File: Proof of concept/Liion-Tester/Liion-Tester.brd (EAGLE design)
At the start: 100 x 80 mm, 24 parts, among them Q2 SI4403DDY-T1-GE3, U1 1042, U2 NCP1854FCCT1G, U3 BQ27427YZFR

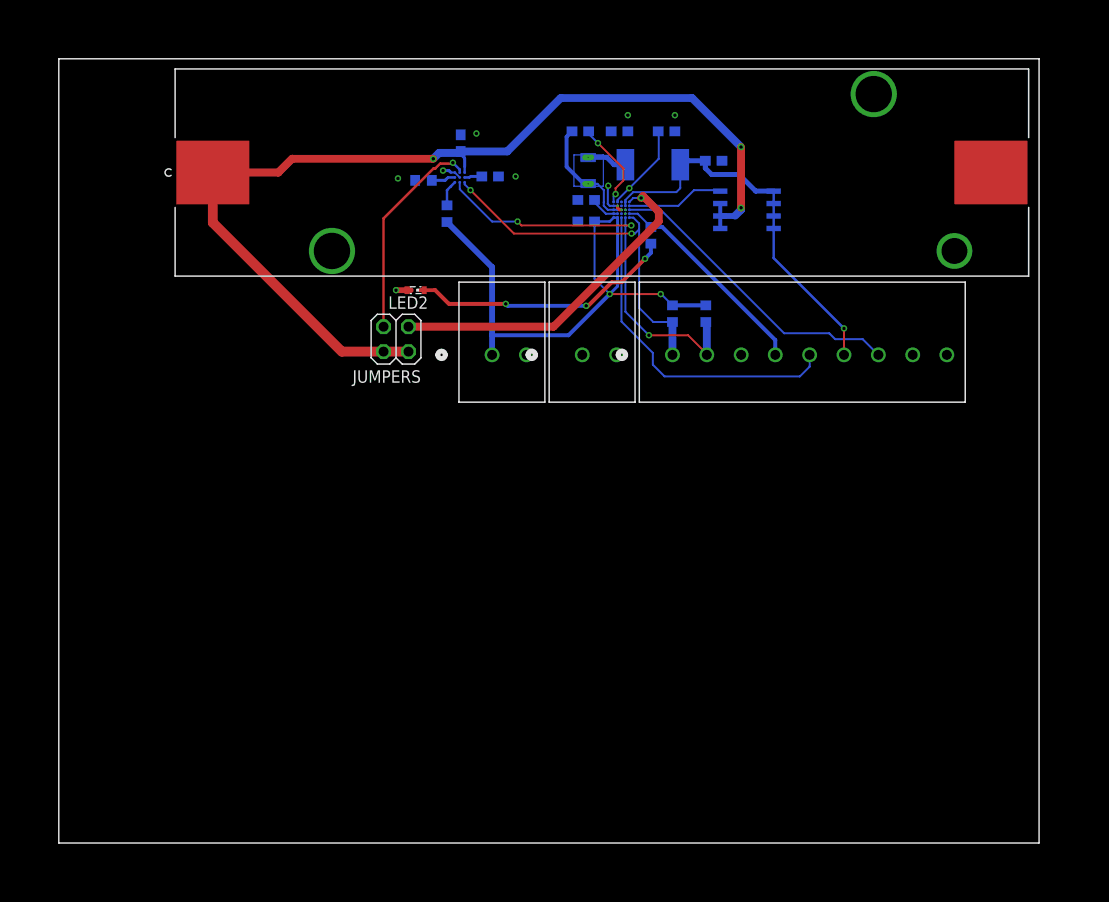
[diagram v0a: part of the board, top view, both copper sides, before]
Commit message: Finished .brd with changes in schematic
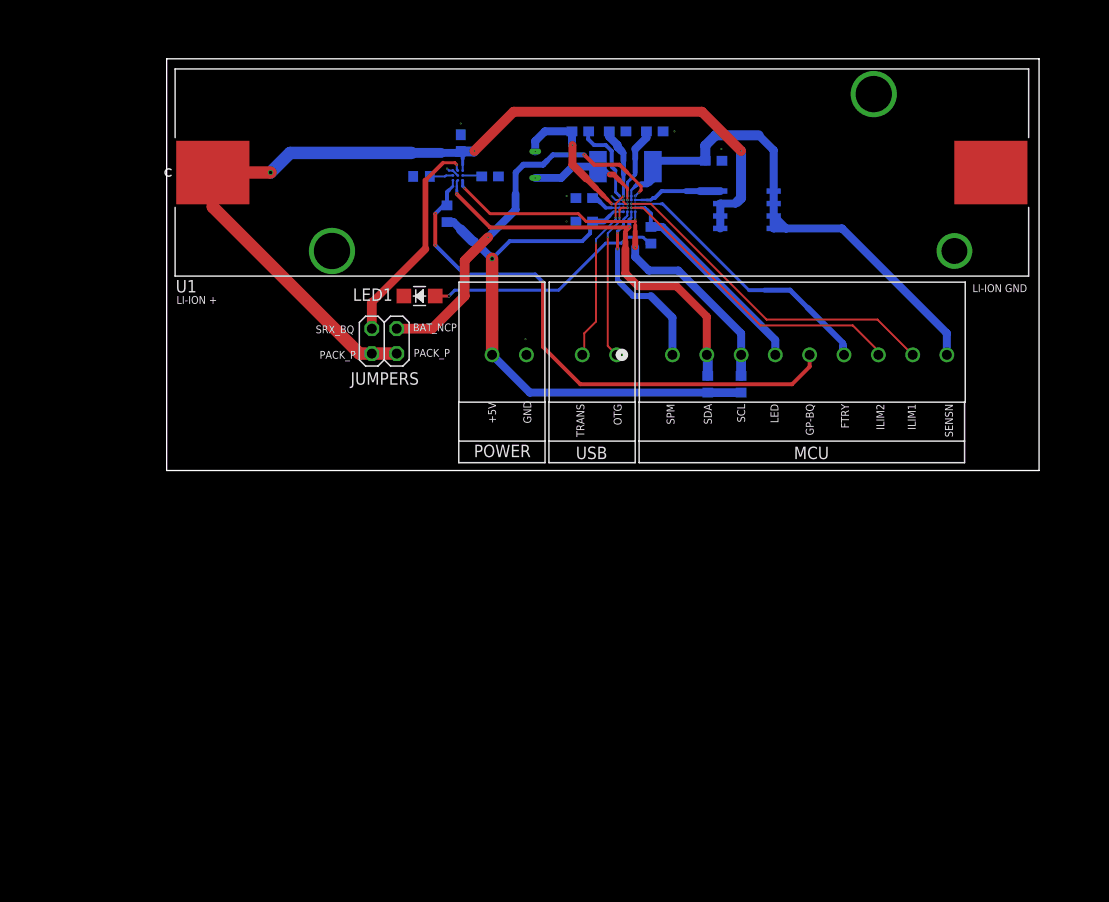
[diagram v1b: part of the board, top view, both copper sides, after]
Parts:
- removed LED2: GREEN, led:SMARTLED-TTW
- added LED1: FYLS-1206PGC, custom_library:LED_QBLP650_1206_QTB
- moved R7 10.0 mm to (69.6, 46.8), turned to 270 degrees
- moved R8 7.20 mm to (66.2, 46.8), turned to 270 degrees
- moved L1 5.43 mm to (48.6, 69.2), turned to 90 degrees
- moved C8 5.00 mm to (57.0, 72.6)
- moved C7 3.60 mm to (60.8, 72.6)
- moved R6 2.81 mm to (57.8, 69.0)
- moved JUMPERS 1.22 mm to (33.2, 51.2)
- moved U2 0.85 mm to (58.0, 65.2)
- moved R1 0.45 mm to (37.0, 68.0)
- moved U3 0.28 mm to (40.7, 68.1)
- moved C4 0.28 mm to (53.6, 65.8)
- moved C3 0.20 mm to (53.6, 63.4)
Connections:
- removed net N$5: LED2.A@1, R5.1
- new net N$4: LED1.2, R5.1
- net FTRY: now also MCU.6; no longer MCU.7
- net GND: now also LED1.1; no longer LED2.C@1
- net GPOUT_BQ: now also MCU.5; no longer MCU.3
- net ILIM2: now also MCU.7; no longer MCU.9
- net OTG: now also USB.2; no longer USB.1
- net SCL: now also MCU.3; no longer MCU.1
- net SENSN: now also MCU.9; no longer MCU.6
- net SPM: now also MCU.1; no longer MCU.5
- net TRANS: now also USB.1; no longer USB.2
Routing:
- net GPOUT_BQ: track 2.68 -> 57.4 mm, vias 0 -> 3
- net ILIM1: track 0.00 -> 35.1 mm
- net ILIM2: track 0.00 -> 31.6 mm
- net N$5: track 27.4 -> 0.00 mm, vias 3 -> 0
- net N$4: track 0.00 -> 24.8 mm, vias 0 -> 1
- net OTG: track 0.00 -> 16.6 mm, vias 0 -> 3
- net TRANS: track 8.96 -> 25.1 mm, vias 1 -> 3
- net SPM: track 34.4 -> 18.4 mm, vias 0 -> 2
- net SENSN: track 40.2 -> 55.6 mm, vias 1 -> 0
- net SENSP: track 4.11 -> 12.0 mm, vias 0 -> 2
- net N$8: track 0.00 -> 7.41 mm
- net SCL: track 37.5 -> 42.7 mm, vias 2 -> 3
- net BAT_NCP: track 34.9 -> 39.2 mm, vias 1 -> 4
- net +5V: track 58.2 -> 62.3 mm, vias 2 -> 1
- net N$7: track 11.8 -> 15.5 mm, vias 0 -> 2
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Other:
- board size 100 x 80 mm -> 89 x 42 mm
- board text added: "+5V"
- board text added: "BAT_NCP"
- board text added: "FTRY"
- board text added: "GND"
- board text added: "GP-BQ"
- board text added: "ILIM1"
- board text added: "ILIM2"
- board text added: "LED"
- board text added: "LI-ION +"
- board text added: "LI-ION GND"
- board text added: "OTG"
- board text added: "PACK_P"
- board text added: "SCL"
- board text added: "SDA"
- board text added: "SENSN"
- board text added: "SPM"
- board text added: "SRX_BQ"
- board text added: "TRANS"
